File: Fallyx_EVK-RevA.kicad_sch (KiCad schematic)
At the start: 3 parts, among them J7 Conn_01x12_Pin, J8 Conn_01x12_Pin, J9 Conn_01x12_Pin

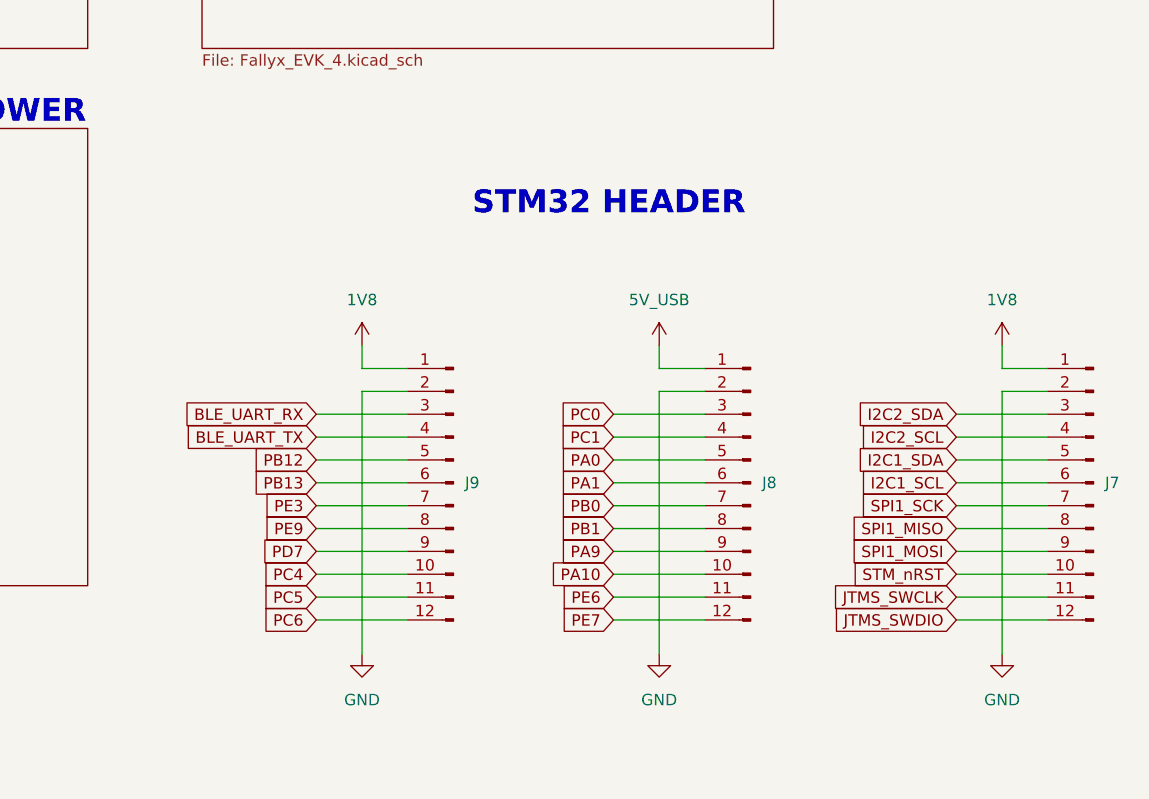
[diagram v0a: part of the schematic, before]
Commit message: review edits
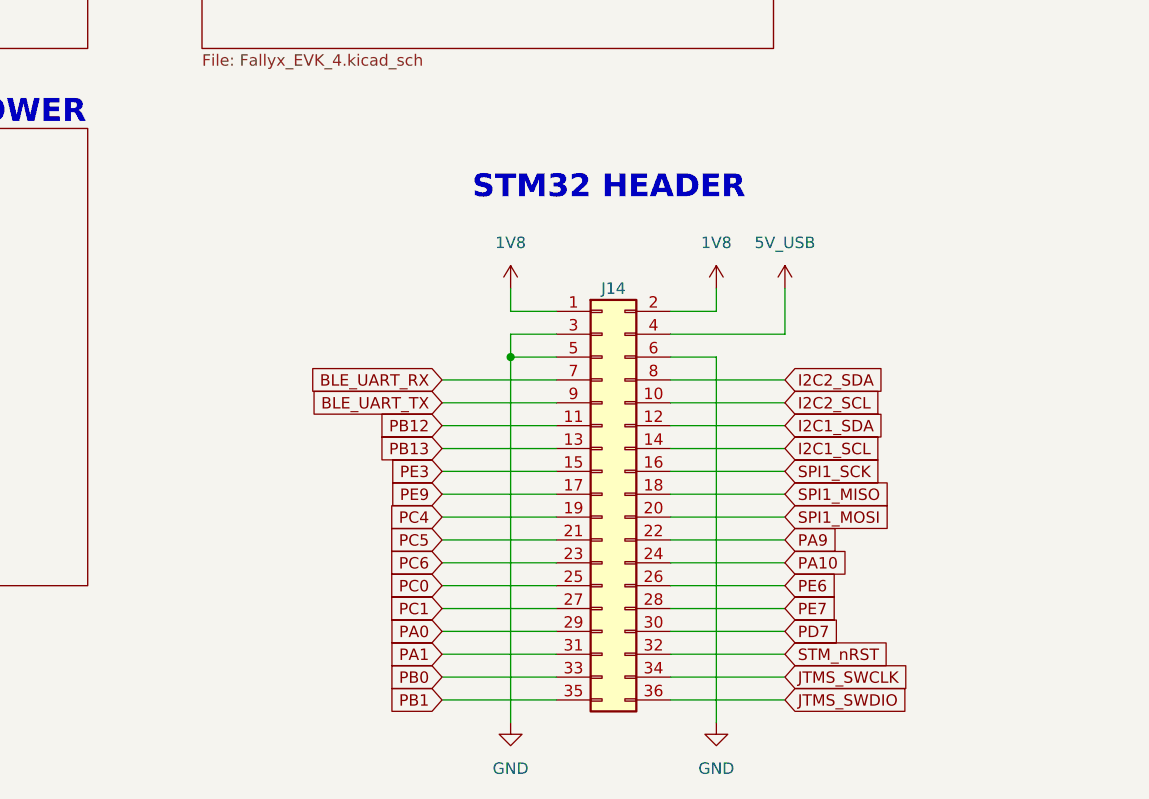
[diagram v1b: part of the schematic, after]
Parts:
- removed J7, J8, J9: Conn_01x12_Pin, Connector_PinHeader_2.54mm:PinHeader_1x12_P2.54mm_Vertical, symbol Connector:Conn_01x12_Pin
- added J14: Conn_02x18_Odd_Even, Connector_PinHeader_2.54mm:PinHeader_2x18_P2.54mm_Vertical, symbol Connector_Generic:Conn_02x18_Odd_Even
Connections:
- net 1V8: now also J14.1 (Pin_1), J14.2 (Pin_2)
- net 5V_USB: now also J14.4 (Pin_4)
- net BLE_UART_RX: now also J14.7 (Pin_7)
- net BLE_UART_TX: now also J14.9 (Pin_9)
- net GND: now also J14.3 (Pin_3), J14.5 (Pin_5), J14.6 (Pin_6)
- net I2C1_SCL: now also J14.14 (Pin_14)
- net I2C1_SDA: now also J14.12 (Pin_12)
- net I2C2_SCL: now also J14.10 (Pin_10)
- net I2C2_SDA: now also J14.8 (Pin_8)
- net JTMS_SWCLK: now also J14.34 (Pin_34)
- net JTMS_SWDIO: now also J14.36 (Pin_36)
- net PA0: now also J14.29 (Pin_29)
- net PA1: now also J14.31 (Pin_31)
- net PA10: now also J14.24 (Pin_24)
- net PA9: now also J14.22 (Pin_22)
- net PB0: now also J14.33 (Pin_33)
- net PB1: now also J14.35 (Pin_35)
- net PB12: now also J14.11 (Pin_11)
- net PB13: now also J14.13 (Pin_13)
- net PC0: now also J14.25 (Pin_25)
- net PC1: now also J14.27 (Pin_27)
- net PC4: now also J14.19 (Pin_19)
- net PC5: now also J14.21 (Pin_21)
- net PC6: now also J14.23 (Pin_23)
- net PD7: now also J14.30 (Pin_30)
- net PE3: now also J14.15 (Pin_15)
- net PE6: now also J14.26 (Pin_26)
- net PE7: now also J14.28 (Pin_28)
- net PE9: now also J14.17 (Pin_17)
- net SPI1_MISO: now also J14.18 (Pin_18)
- net SPI1_MOSI: now also J14.20 (Pin_20)
- net SPI1_SCK: now also J14.16 (Pin_16)
- net STM_nRST: now also J14.32 (Pin_32)
